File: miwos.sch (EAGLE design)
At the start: 50 parts, among them J1 614004190021, U1 PEC16, U3 PEC16

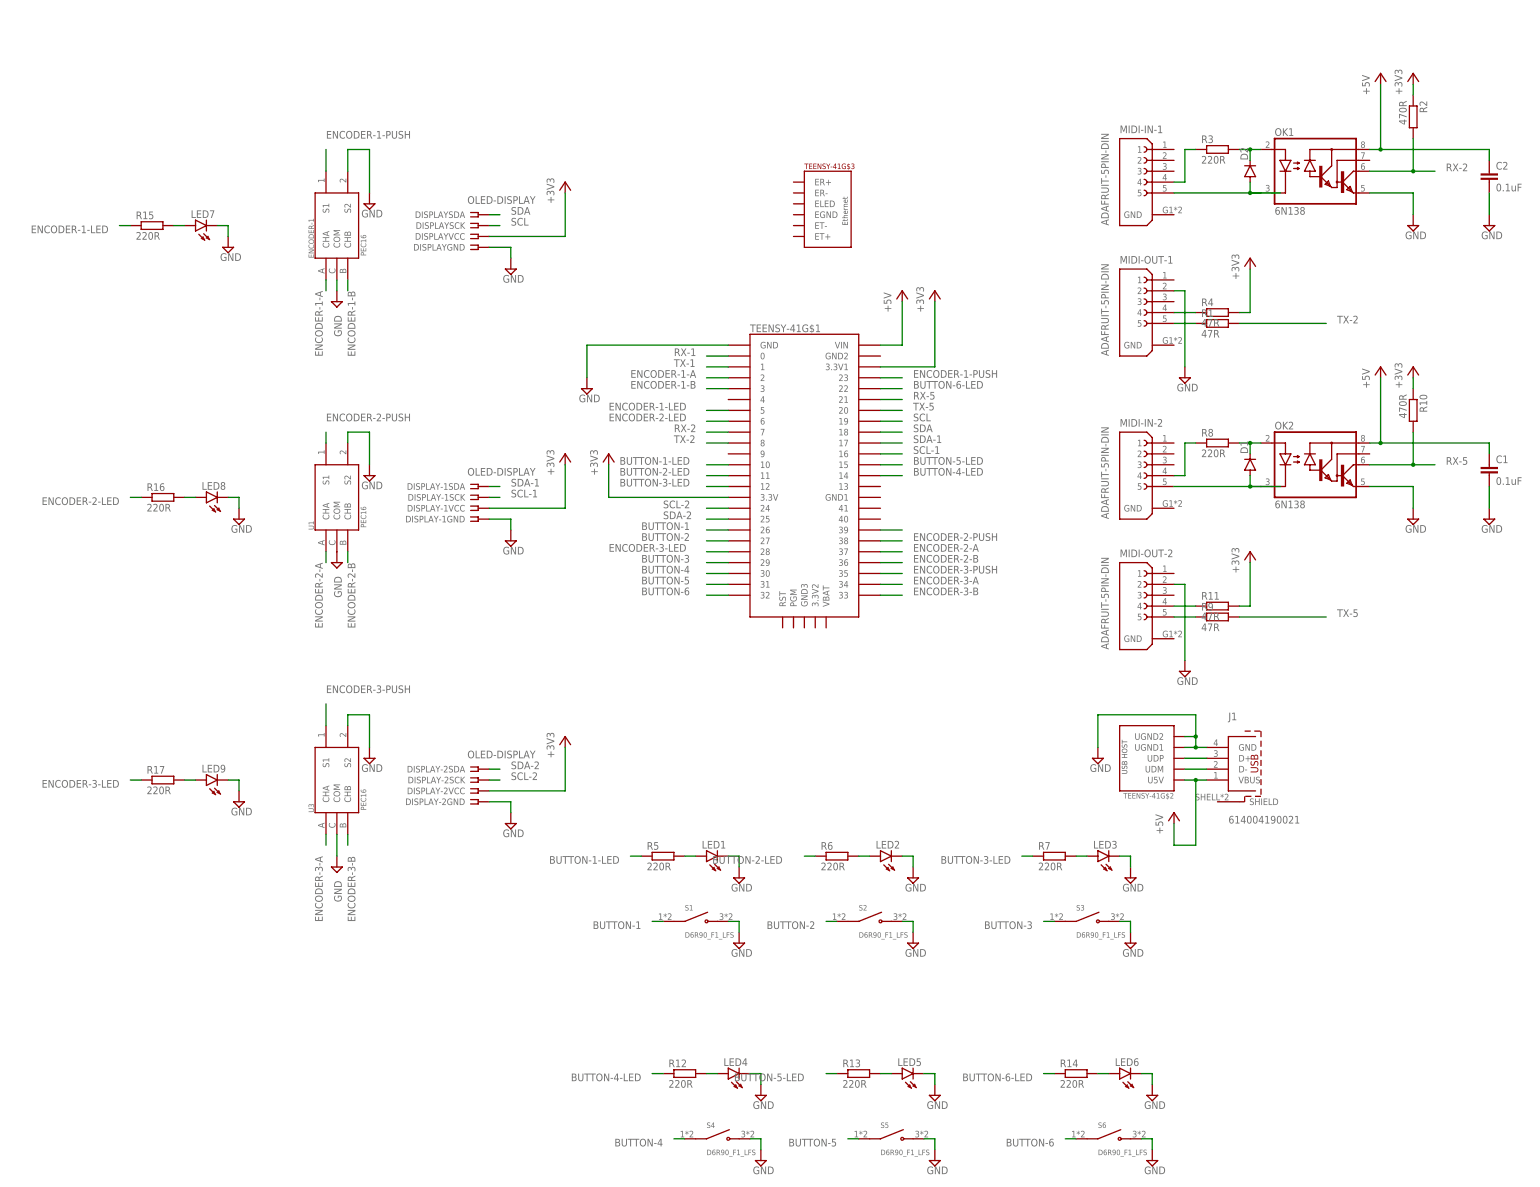
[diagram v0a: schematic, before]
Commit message: Place labels, small fixes
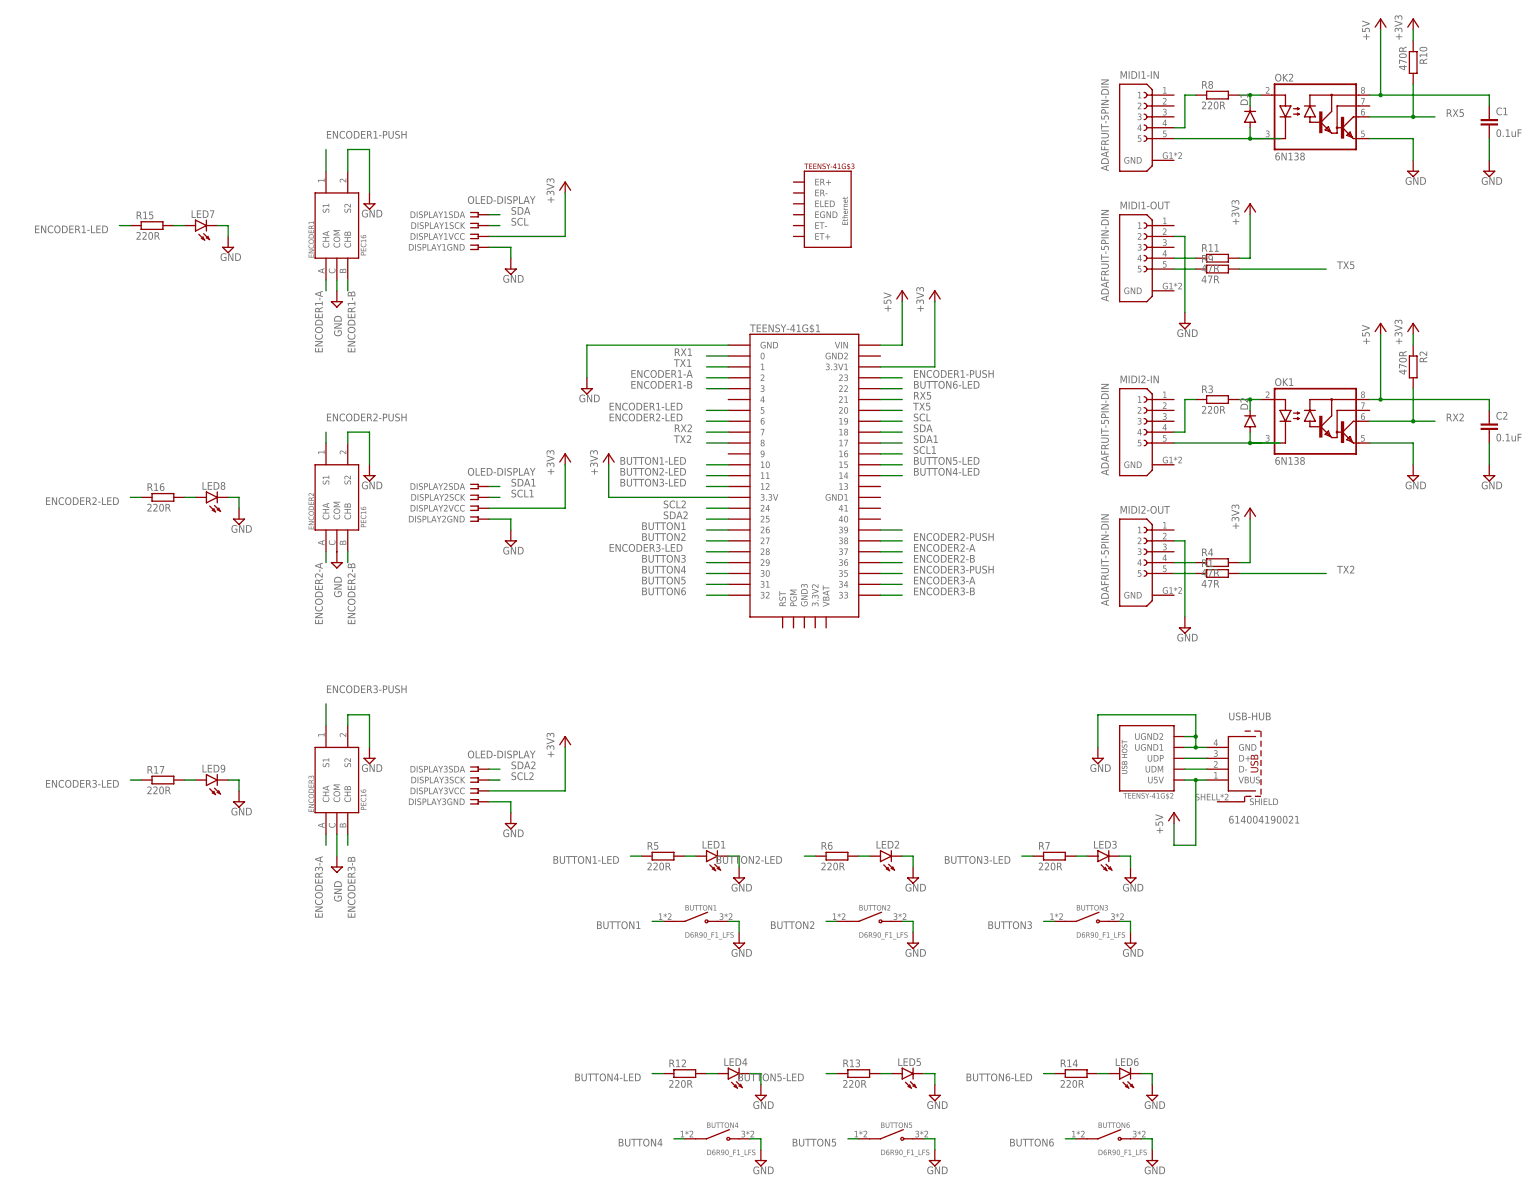
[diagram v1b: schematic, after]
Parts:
- removed MIDI-IN-1, MIDI-IN-2, MIDI-OUT-1, MIDI-OUT-2: ADAFRUIT-5PIN-DIN, adafruit-5pin-din:ADAFRUIT-5PIN-DIN
- added MIDI1-IN, MIDI1-OUT, MIDI2-IN, MIDI2-OUT: ADAFRUIT-5PIN-DIN, adafruit-5pin-din:ADAFRUIT-5PIN-DIN
- renumbered DISPLAY to DISPLAY1, DISPLAY-1 to DISPLAY2, DISPLAY-2 to DISPLAY3, ENCODER-1 to ENCODER1, J1 to USB-HUB, S1 to BUTTON1, S2 to BUTTON2, S3 to BUTTON3, S4 to BUTTON4, S5 to BUTTON5, S6 to BUTTON6, U1 to ENCODER2, U3 to ENCODER3
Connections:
- net BUTTON-1 renamed BUTTON1
- net BUTTON-1-LED renamed BUTTON1-LED
- net BUTTON-2 renamed BUTTON2
- net BUTTON-2-LED renamed BUTTON2-LED
- net BUTTON-3 renamed BUTTON3
- net BUTTON-3-LED renamed BUTTON3-LED
- net BUTTON-4 renamed BUTTON4
- net BUTTON-4-LED renamed BUTTON4-LED
- net BUTTON-5 renamed BUTTON5
- net BUTTON-5-LED renamed BUTTON5-LED
- net BUTTON-6 renamed BUTTON6
- net BUTTON-6-LED renamed BUTTON6-LED
- net ENCODER-1-A renamed ENCODER1-A
- net ENCODER-1-B renamed ENCODER1-B
- net ENCODER-1-LED renamed ENCODER1-LED
- net ENCODER-1-PUSH renamed ENCODER1-PUSH
- net ENCODER-2-A renamed ENCODER2-A
- net ENCODER-2-B renamed ENCODER2-B
- net ENCODER-2-LED renamed ENCODER2-LED
- net ENCODER-2-PUSH renamed ENCODER2-PUSH
- net ENCODER-3-A renamed ENCODER3-A
- net ENCODER-3-B renamed ENCODER3-B
- net ENCODER-3-LED renamed ENCODER3-LED
- net ENCODER-3-PUSH renamed ENCODER3-PUSH
- net RX-1 renamed RX1
- net RX-2 renamed RX2
- net RX-5 renamed RX5
- net SCL-1 renamed SCL1
- net SCL-2 renamed SCL2
- net SDA-1 renamed SDA1
- net SDA-2 renamed SDA2
- net TX-1 renamed TX1
- net TX-2 renamed TX2
- net TX-5 renamed TX5
- net GND: now also MIDI1-OUT.2, MIDI2-OUT.2; no longer MIDI-OUT-1.2, MIDI-OUT-2.2
- net N$10: now also MIDI1-IN.4; no longer MIDI-IN-2.4
- net N$11: now also MIDI1-OUT.5; no longer MIDI-OUT-2.5
- net N$12: now also MIDI1-OUT.4; no longer MIDI-OUT-2.4
- net N$17: now also MIDI2-IN.5; no longer MIDI-IN-1.5
- net N$18: now also MIDI2-IN.4; no longer MIDI-IN-1.4
- net N$19: now also MIDI2-OUT.5; no longer MIDI-OUT-1.5
- net N$21: now also MIDI2-OUT.4; no longer MIDI-OUT-1.4
- net N$9: now also MIDI1-IN.5; no longer MIDI-IN-2.5
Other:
- moved on the sheet: C1, C2, D1, D2, OK1, OK2, R1, R10, R11, R2, R3, R4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
